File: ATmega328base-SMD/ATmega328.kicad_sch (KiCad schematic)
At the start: 11 parts, among them J1 FTDI, J2 Power in, U1 AMS1117-5_0, U2 ATMEGA328P-AU, X1 X322516MLB4SI

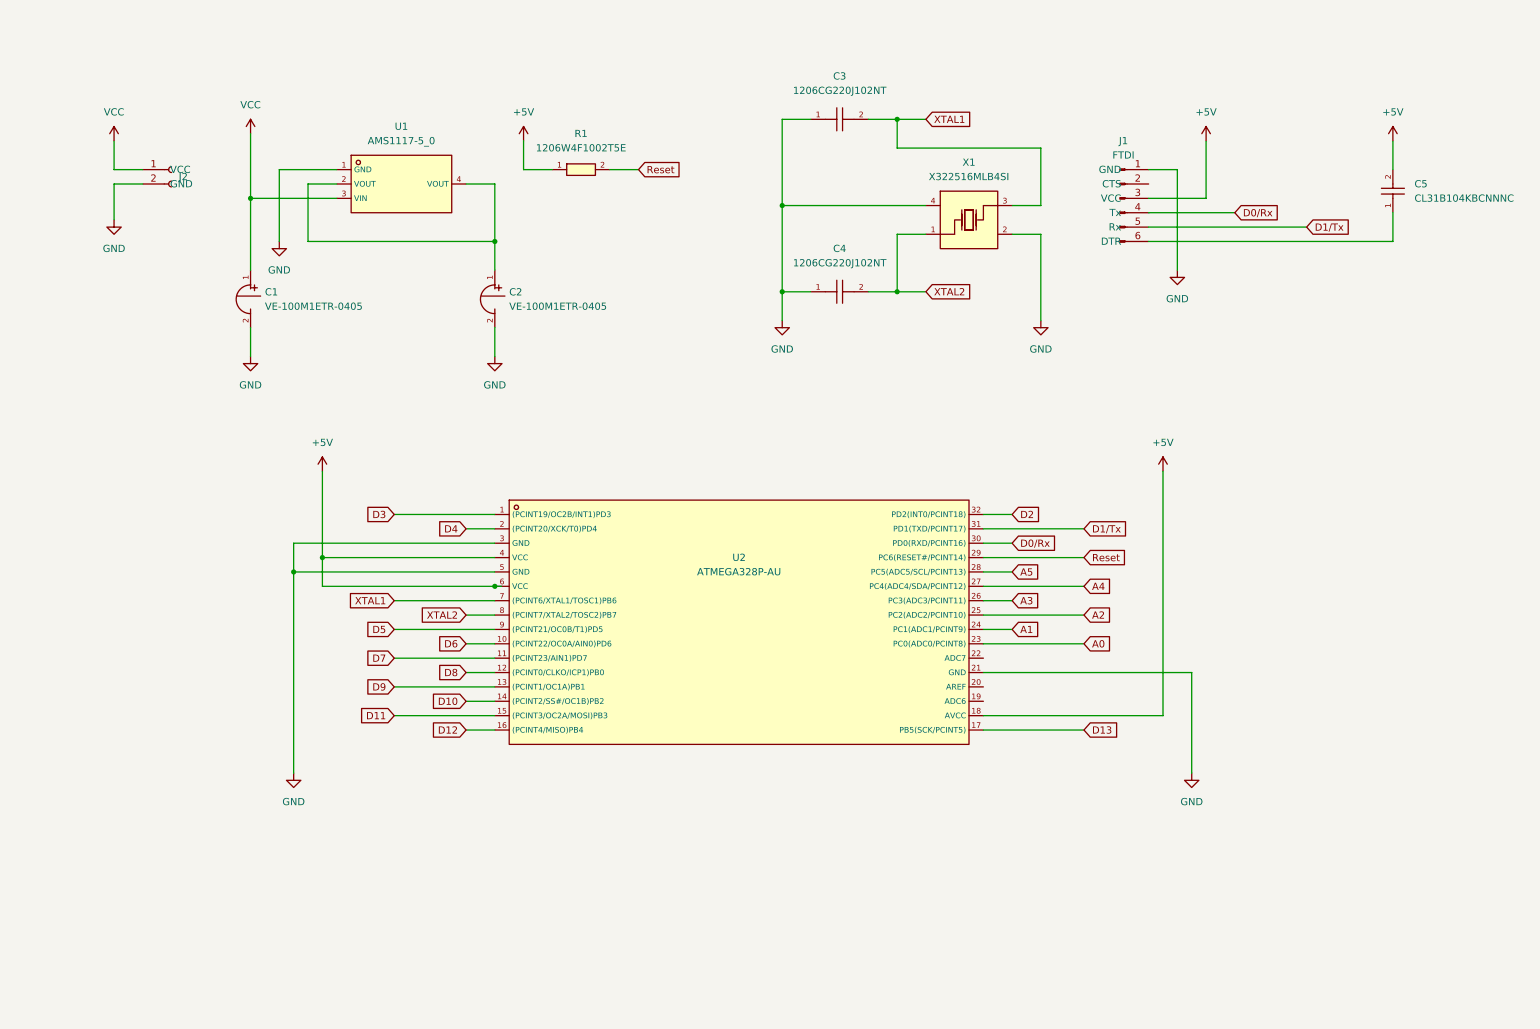
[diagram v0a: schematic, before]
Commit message: atmega base
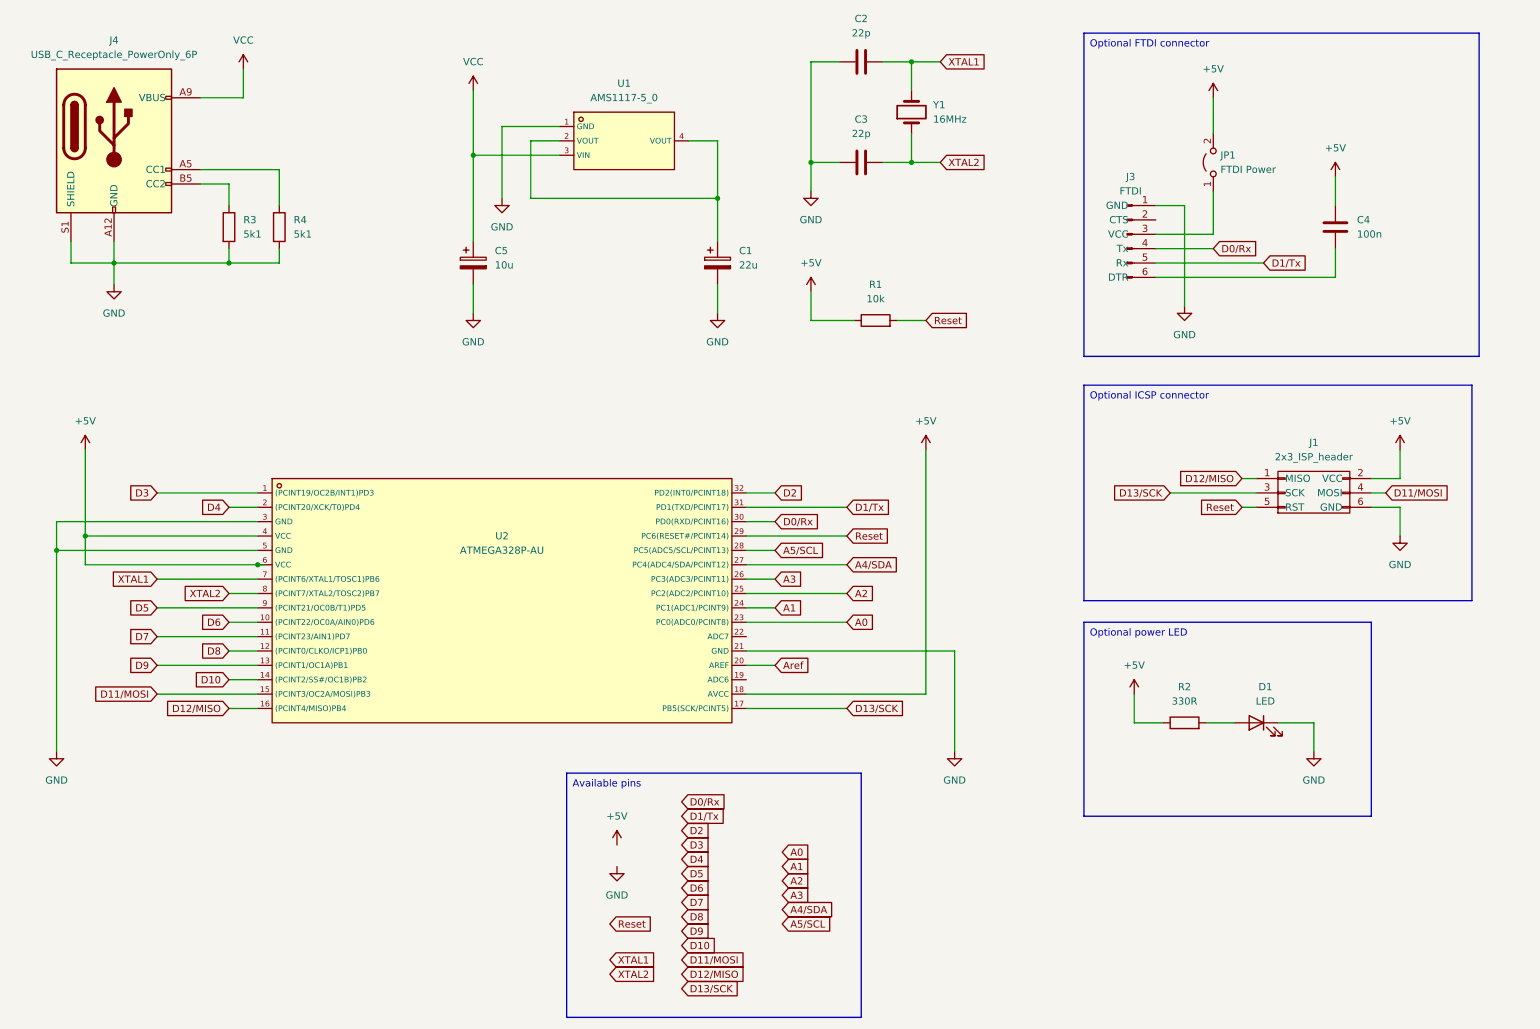
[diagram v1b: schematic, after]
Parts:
- removed C1, C2: VE-100M1ETR-0405, JLC2KiCad_Footprints:CAP-SMD_BD4.0-L4.3-W4.3-RD, symbol JLC2KiCad_Symbols:VE-100M1ETR-0405
- removed C3, C4: 1206CG220J102NT, JLC2KiCad_Footprints:C1206, symbol JLC2KiCad_Symbols:1206CG220J102NT
- removed C5: CL31B104KBCNNNC, JLC2KiCad_Footprints:C1206, symbol JLC2KiCad_Symbols:CL31B104KBCNNNC
- removed J1: FTDI, My_Headers:6-pin FTDI Programmer PinSocket large, symbol My_Headers:6-pin_FTDI_header
- removed J2: Power in, My_Misc:BarrelJack_Horizontal, symbol My_Headers:2-pin_power_input_header
- removed R1: 1206W4F1002T5E, JLC2KiCad_Footprints:R1206, symbol JLC2KiCad_Symbols:1206W4F1002T5E
- removed X1: X322516MLB4SI, JLC2KiCad_Footprints:OSC-SMD_4P-L3.2-W2.5-BL, symbol JLC2KiCad_Symbols:X322516MLB4SI
- added C1: 22u, Capacitor_SMD:CP_Elec_4x5.3, symbol Device:C_Polarized
- added C2, C3: 22p, Capacitor_SMD:C_1206_3216Metric_Pad1.33x1.80mm_HandSolder, symbol Device:C
- added C4: 100n, Capacitor_SMD:C_1206_3216Metric_Pad1.33x1.80mm_HandSolder, symbol Device:C
- added C5: 10u, Capacitor_SMD:CP_Elec_5x5.4, symbol Device:C_Polarized
- added D1: LED, LED_SMD:LED_1206_3216Metric_Pad1.42x1.75mm_HandSolder, symbol Device:LED
- added J1: 2x3_ISP_header, Connector_PinHeader_2.54mm:PinHeader_2x03_P2.54mm_Vertical_SMD, symbol My_Headers:2x3_ISP_header
- added J3: FTDI, Connector_PinHeader_2.54mm:PinHeader_1x06_P2.54mm_Vertical_SMD_Pin1Left, symbol My_Headers:6-pin_FTDI_header
- added J4: USB_C_Receptacle_PowerOnly_6P, Connector_USB:USB_C_Receptacle_GCT_USB4135-GF-A_6P_TopMnt_Horizontal, symbol Connector:USB_C_Receptacle_PowerOnly_6P
- added JP1: FTDI Power, Button_Switch_SMD:SW_DIP_SPSTx01_Slide_6.7x4.1mm_W6.73mm_P2.54mm_LowProfile_JPin, symbol Jumper:Jumper_2_Open
- added R1: 10k, Resistor_SMD:R_1206_3216Metric_Pad1.30x1.75mm_HandSolder, symbol Device:R
- added R2: 330R, Resistor_SMD:R_1206_3216Metric_Pad1.30x1.75mm_HandSolder, symbol Device:R
- added R3, R4: 5k1, Resistor_SMD:R_1206_3216Metric_Pad1.30x1.75mm_HandSolder, symbol Device:R
- added Y1: 16MHz, Crystal:Crystal_SMD_HC49-SD, symbol Device:Crystal
- U1: footprint JLC2KiCad_Footprints:SOT-223_L6.5-W3.5-P2.30-LS7.0-BR -> Package_TO_SOT_SMD:SOT-223
- U2: footprint JLC2KiCad_Footprints:TQFP-32_L7.0-W7.0-P0.80-LS9.0-BL -> Package_QFP:TQFP-32_7x7mm_P0.8mm
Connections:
- net +5V: now also C4.1, J1.2 (VCC), JP1.2 (B), R1.1, R2.1
- net D0/Rx: now also J3.4 (Tx)
- net D1/Tx: now also J3.5 (Rx)
- net GND: now also C1.2, C2.1, C3.1, C5.2, D1.1 (K), J1.6 (GND), J3.1 (GND), J4.A12 (GND), J4.B12 (GND), J4.S1 (SHIELD), R3.2, R4.2
- net Reset: now also J1.5 (RST), R1.2
- net VCC: now also C5.1, J4.A9 (VBUS), J4.B9 (VBUS)
- net XTAL1: now also C2.2, Y1.2
- net XTAL2: now also C3.2, Y1.1
- net Aref: now reaches U2.20 (AREF)
- net at U1.2 (VOUT), U1.4 (VOUT): now also C1.1
- net A4 renamed A4/SDA
- net A5 renamed A5/SCL
- net D11 renamed D11/MOSI
- net D11/MOSI: now also J1.4 (MOSI)
- net D12 renamed D12/MISO
- net D12/MISO: now also J1.1 (MISO)
- net D13 renamed D13/SCK
- net D13/SCK: now also J1.3 (SCK)
- new net: D1.2 (A), R2.2
- new net: J3.3 (VCC), JP1.1 (A)
- new net: C4.2, J3.6 (DTR)
- new net: J4.A5 (CC1), R4.1
- new net: J4.B5 (CC2), R3.1
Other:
- moved on the sheet: U1, U2
